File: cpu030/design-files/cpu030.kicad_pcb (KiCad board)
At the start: 4 copper layers, 106 parts, among them J101 Reset, J102 SYSCTL JTAG, J103 NMI, J201 DRAM0SZ, J202 DRAM0 JTAG, J301 UART0 FTDI, J302 UART1 FTDI, J303 UART1, J304 UART0, SW101 Reset, SW102 NMI, U101 MC68030RC, U102 ATF1508AS, U103 MC74ACT05DG, U104 DS1813, U105 SST39SF040 (E), U106 SST39SF040 (O), U107 MC68882, U108 GAL22V10, U109 MC74ACT05DG, U110 DS1813, U201 ATF1508AS, U202 CY7C1061GE (U16), U203 CY7C1061GE (L16), U204 SIMM72-0A, U205 SIMM72-0B, U206 MC74ACT05DG, U301 TL16C2552, Y101 50MHz, Y301 1.8432MHz

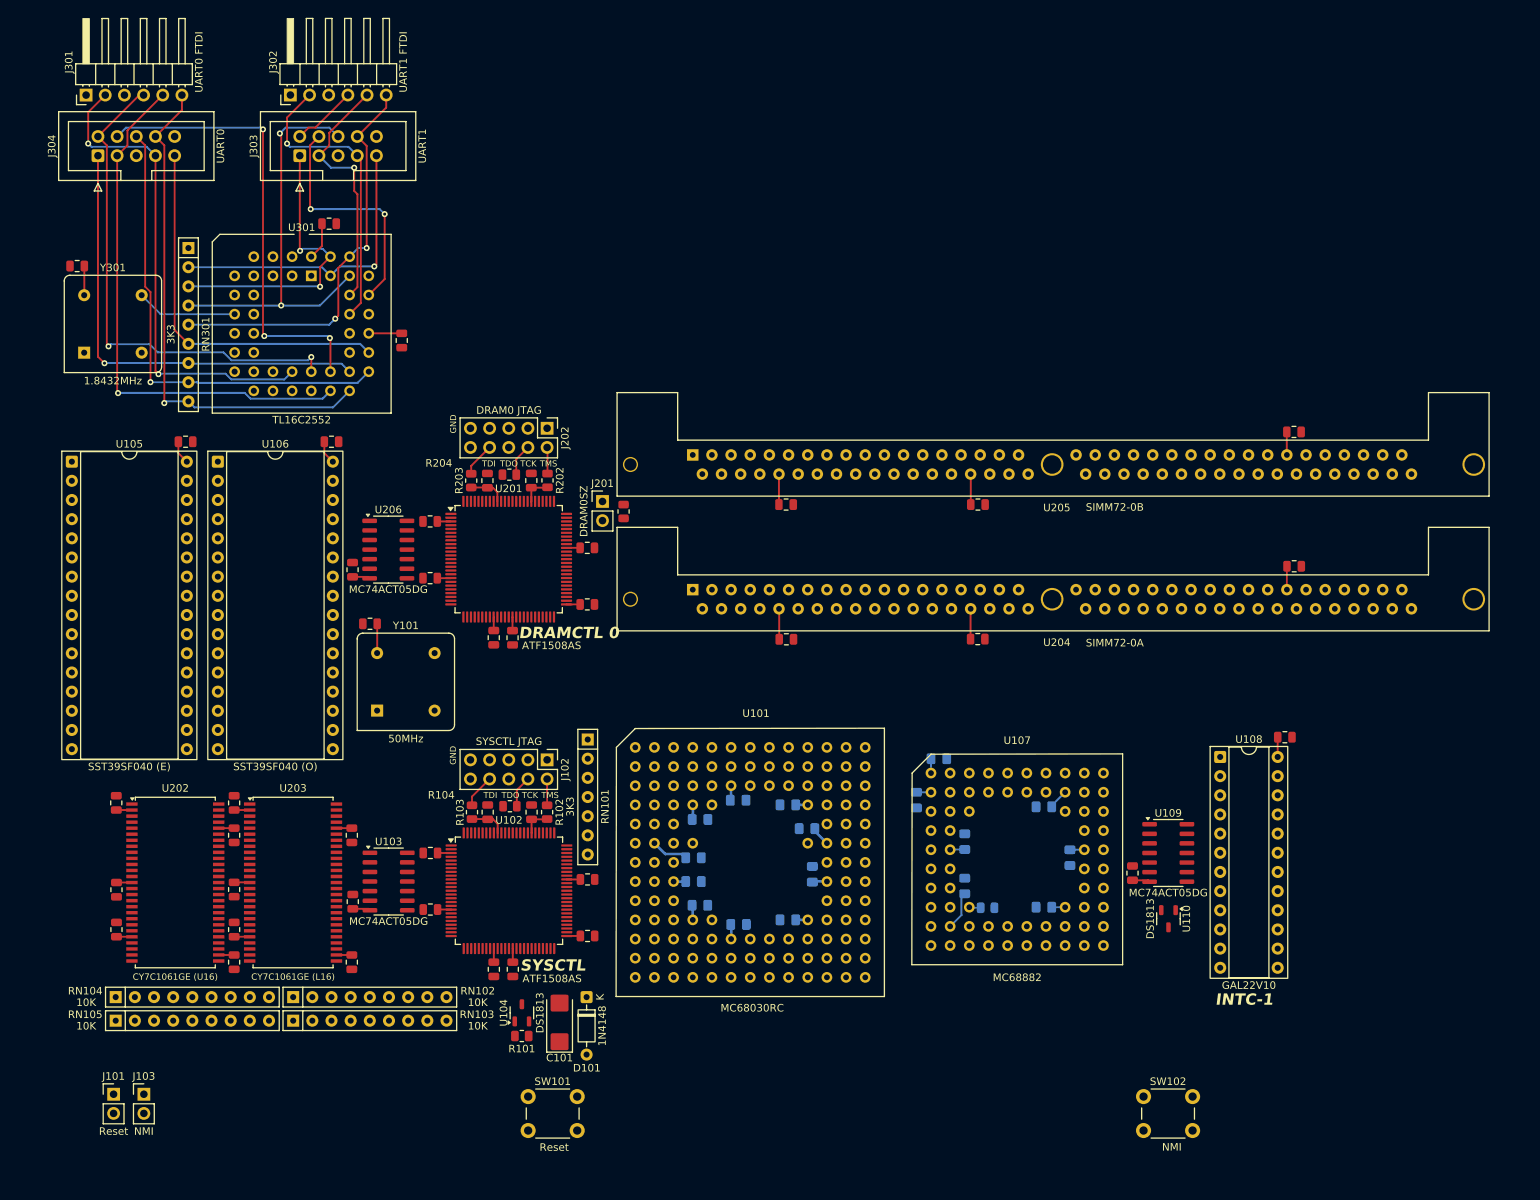
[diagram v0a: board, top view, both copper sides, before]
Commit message: System timer.
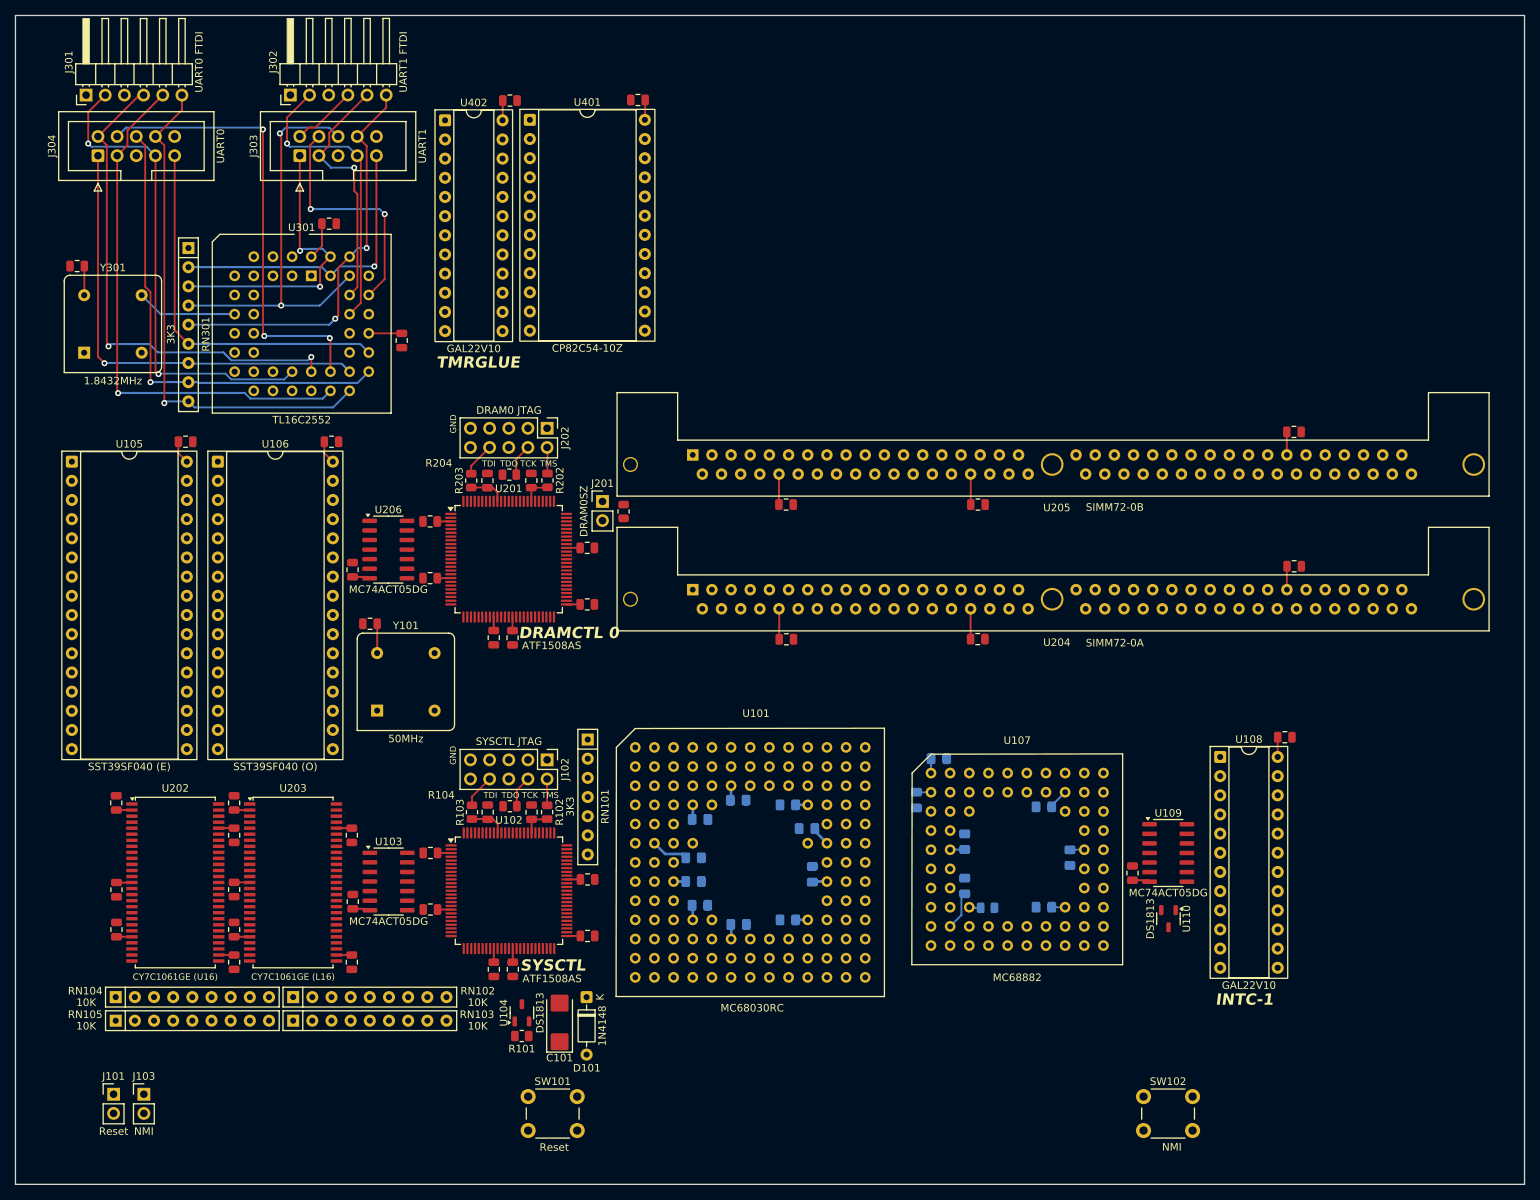
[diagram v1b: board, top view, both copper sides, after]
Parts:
- added C401: 100nF, Capacitor_SMD:C_0805_2012Metric, F.Cu at (228.7, 95.6)
- added C402: 100nF, Capacitor_SMD:C_0805_2012Metric, F.Cu at (211.8, 95.7)
- added U401: CP82C54-10Z, Package_DIP:DIP-24_W15.24mm_Socket, F.Cu at (214.4, 98.2)
- added U402: GAL22V10, Package_DIP:DIP-24_W7.62mm_Socket, F.Cu at (203.2, 98.3)
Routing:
- net +5V: track 154.8 -> 160.1 mm
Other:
- board outline added: 200 x 154.9 mm
- board text added: "TMRGLUE"

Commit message: Eliminate the external D-FF clocking on INTC-1; use the same trick with /DS as we do on TMRGLUE.
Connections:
- U108 pad 1: Net-(U108-I1/CLK) -> ~{DS}
- U108 pad 13: ~{DS} -> RnW
- U108 pad 14: RnW -> unconnected-(U108-IO1-Pad14)
- U108 pad 23: Net-(U108-I1/CLK) -> unconnected-(U108-IO10-Pad23)
- U109 pad 5: GND -> TMR_O0
- U109 pad 6: unconnected-(U109-Pad6) -> ~{INT6}
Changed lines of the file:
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@@
 	(net 251 "Net-(U107-A0)")
 	(net 252 "~{INT5}")
-	(net 253 "Net-(U108-I1{slash}CLK)")
-	(net 254 "~{INT1}")
-	(net 255 "~{INT7}")
-	(net 256 "~{INT6}")
-	(net 257 "~{INT2}")
-	(net 258 "~{INT4}")
-	(net 259 "~{INT3}")
-	(net 260 "unconnected-(U108-IO9-Pad22)")
-	(net 261 "unconnected-(U109-Pad10)")
-	(net 262 "unconnected-(U109-Pad8)")
-	(net 263 "unconnected-(U109-Pad6)")
-	(net 264 "unconnected-(U109-Pad12)")
-	(net 265 "Net-(U401-OUT0)")
-	(net 266 "Net-(U401-G2)")
-	(net 267 "Net-(U401-~{CS})")
-	(net 268 "Net-(U401-OUT2)")
-	(net 269 "Net-(U401-G1)")
-	(net 270 "Net-(U401-OUT1)")
-	(net 271 "Net-(U401-G0)")
-	(net 272 "unconnected-(U402-I8-Pad8)")
-	(net 273 "unconnected-(U402-I11-Pad11)")
-	(net 274 "unconnected-(U402-I9-Pad9)")
-	(net 275 "TMR_O2")
-	(net 276 "unconnected-(U402-I10-Pad10)")
-	(net 277 "TMR_O0")
-	(net 278 "TMR_O1")
+	(net 253 "~{INT1}")
+	(net 254 "~{INT7}")
+	(net 255 "~{INT6}")
+	(net 256 "~{INT2}")
+	(net 257 "~{INT4}")
+	(net 258 "~{INT3}")
+	(net 259 "unconnected-(U108-IO9-Pad22)")
+	(net 260 "unconnected-(U109-Pad10)")
+	(net 261 "unconnected-(U109-Pad8)")
+	(net 262 "unconnected-(U109-Pad12)")
+	(net 263 "Net-(U401-OUT0)")
+	(net 264 "Net-(U401-G2)")
+	(net 265 "Net-(U401-~{CS})")
+	(net 266 "Net-(U401-OUT2)")
+	(net 267 "Net-(U401-G1)")
+	(net 268 "Net-(U401-OUT1)")
+	(net 269 "Net-(U401-G0)")
+	(net 270 "unconnected-(U402-I8-Pad8)")
+	(net 271 "unconnected-(U402-I11-Pad11)")
+	(net 272 "unconnected-(U402-I9-Pad9)")
+	(net 273 "TMR_O2")
+	(net 274 "unconnected-(U402-I10-Pad10)")
+	(net 275 "TMR_O0")
+	(net 276 "TMR_O1")
+	(net 277 "unconnected-(U108-IO1-Pad14)")
+	(net 278 "unconnected-(U108-IO10-Pad23)")
 	(footprint "Package_QFP:TQFP-100_14x14mm_P0.5mm"
 		(layer "F.Cu")
@@
 			(layers "*.Cu" "*.Mask")
 			(remove_unused_layers no)
-			(net 265 "Net-(U401-OUT0)")
+			(net 263 "Net-(U401-OUT0)")
 			(pinfunction "I5")
 			(pintype "input")
@@
 			(layers "*.Cu" "*.Mask")
 			(remove_unused_layers no)
-			(net 270 "Net-(U401-OUT1)")
+			(net 268 "Net-(U401-OUT1)")
 			(pinfunction "I6")
 			(pintype "input")
@@
 			(layers "*.Cu" "*.Mask")
 			(remove_unused_layers no)
-			(net 268 "Net-(U401-OUT2)")
+			(net 266 "Net-(U401-OUT2)")
 			(pinfunction "I7")
 			(pintype "input")
@@
 			(layers "*.Cu" "*.Mask")
 			(remove_unused_layers no)
-			(net 272 "unconnected-(U402-I8-Pad8)")
+			(net 270 "unconnected-(U402-I8-Pad8)")
 			(pinfunction "I8")
 			(pintype "input+no_connect")
@@
 			(layers "*.Cu" "*.Mask")
 			(remove_unused_layers no)
-			(net 274 "unconnected-(U402-I9-Pad9)")
+			(net 272 "unconnected-(U402-I9-Pad9)")
 			(pinfunction "I9")
 			(pintype "input+no_connect")
@@
 			(layers "*.Cu" "*.Mask")
 			(remove_unused_layers no)
-			(net 276 "unconnected-(U402-I10-Pad10)")
+			(net 274 "unconnected-(U402-I10-Pad10)")
 			(pinfunction "I10")
 			(pintype "input+no_connect")
@@
 			(layers "*.Cu" "*.Mask")
 			(remove_unused_layers no)
-			(net 273 "unconnected-(U402-I11-Pad11)")
+			(net 271 "unconnected-(U402-I11-Pad11)")
 			(pinfunction "I11")
 			(pintype "input+no_connect")
@@
 			(layers "*.Cu" "*.Mask")
 			(remove_unused_layers no)
-			(net 277 "TMR_O0")
+			(net 275 "TMR_O0")
 			(pinfunction "IO4")
 			(pintype "tri_state")
@@
 			(layers "*.Cu" "*.Mask")
 			(remove_unused_layers no)
-			(net 278 "TMR_O1")
+			(net 276 "TMR_O1")
 			(pinfunction "IO5")
 			(pintype "tri_state")
@@
 			(layers "*.Cu" "*.Mask")
 			(remove_unused_layers no)
-			(net 275 "TMR_O2")
+			(net 273 "TMR_O2")
 			(pinfunction "IO6")
 			(pintype "tri_state")
@@
 			(layers "*.Cu" "*.Mask")
 			(remove_unused_layers no)
-			(net 271 "Net-(U401-G0)")
+			(net 269 "Net-(U401-G0)")
 			(pinfunction "IO7")
 			(pintype "tri_state")
@@
 			(layers "*.Cu" "*.Mask")
 			(remove_unused_layers no)
-			(net 269 "Net-(U401-G1)")
+			(net 267 "Net-(U401-G1)")
 			(pinfunction "IO8")
 			(pintype "tri_state")
@@
 			(layers "*.Cu" "*.Mask")
 			(remove_unused_layers no)
-			(net 266 "Net-(U401-G2)")
+			(net 264 "Net-(U401-G2)")
 			(pinfunction "IO9")
 			(pintype "tri_state")
@@
 			(layers "*.Cu" "*.Mask")
 			(remove_unused_layers no)
-			(net 267 "Net-(U401-~{CS})")
+			(net 265 "Net-(U401-~{CS})")
 			(pinfunction "IO10")
 			(pintype "tri_state")
@@
 			(layers "*.Cu" "*.Mask")
 			(remove_unused_layers no)
-			(net 265 "Net-(U401-OUT0)")
+			(net 263 "Net-(U401-OUT0)")
 			(pinfunction "OUT0")
 			(pintype "output")
@@
 			(layers "*.Cu" "*.Mask")
 			(remove_unused_layers no)
-			(net 271 "Net-(U401-G0)")
+			(net 269 "Net-(U401-G0)")
 			(pinfunction "G0")
 			(pintype "input")
@@
 			(layers "*.Cu" "*.Mask")
 			(remove_unused_layers no)
-			(net 270 "Net-(U401-OUT1)")
+			(net 268 "Net-(U401-OUT1)")
 			(pinfunction "OUT1")
 			(pintype "output")
@@
 			(layers "*.Cu" "*.Mask")
 			(remove_unused_layers no)
-			(net 269 "Net-(U401-G1)")
+			(net 267 "Net-(U401-G1)")
 			(pinfunction "G1")
 			(pintype "input")
@@
 			(layers "*.Cu" "*.Mask")
 			(remove_unused_layers no)
-			(net 266 "Net-(U401-G2)")
+			(net 264 "Net-(U401-G2)")
 			(pinfunction "G2")
 			(pintype "input")
@@
 			(layers "*.Cu" "*.Mask")
 			(remove_unused_layers no)
-			(net 268 "Net-(U401-OUT2)")
+			(net 266 "Net-(U401-OUT2)")
 			(pinfunction "OUT2")
 			(pintype "output")
@@
 			(layers "*.Cu" "*.Mask")
 			(remove_unused_layers no)
-			(net 267 "Net-(U401-~{CS})")
+			(net 265 "Net-(U401-~{CS})")
 			(pinfunction "~{CS}")
 			(pintype "input")
@@
 			(layers "F.Cu" "F.Mask" "F.Paste")
 			(roundrect_rratio 0.25)
-			(net 11 "GND")
+			(net 275 "TMR_O0")
 			(pintype "input")
 		)
@@
 			(layers "F.Cu" "F.Mask" "F.Paste")
 			(roundrect_rratio 0.25)
-			(net 263 "unconnected-(U109-Pad6)")
-			(pintype "open_collector+no_connect")
+			(net 255 "~{INT6}")
+			(pintype "open_collector")
 		)
 		(pad "7" smd roundrect
@@
 			(layers "F.Cu" "F.Mask" "F.Paste")
 			(roundrect_rratio 0.25)
-			(net 262 "unconnected-(U109-Pad8)")
+			(net 261 "unconnected-(U109-Pad8)")
 			(pintype "open_collector+no_connect")
 		)
@@
 			(layers "F.Cu" "F.Mask" "F.Paste")
 			(roundrect_rratio 0.25)
-			(net 261 "unconnected-(U109-Pad10)")
+			(net 260 "unconnected-(U109-Pad10)")
 			(pintype "open_collector+no_connect")
 		)
@@
 			(layers "F.Cu" "F.Mask" "F.Paste")
 			(roundrect_rratio 0.25)
-			(net 264 "unconnected-(U109-Pad12)")
+			(net 262 "unconnected-(U109-Pad12)")
 			(pintype "open_collector+no_connect")
 		)
@@
 			(layers "*.Cu" "*.Mask")
 			(remove_unused_layers no)
-			(net 255 "~{INT7}")
+			(net 254 "~{INT7}")
 			(pinfunction "1")
 			(pintype "passive")
@@
 			(layers "*.Cu" "*.Mask")
 			(remove_unused_layers no)
-			(net 255 "~{INT7}")
+			(net 254 "~{INT7}")
 			(pinfunction "1")
 			(pintype "passive")
@@
 			(remove_unused_layers no)
 			(roundrect_rratio 0.15625)
-			(net 253 "Net-(U108-I1{slash}CLK)")
+			(net 86 "~{DS}")
 			(pinfunction "I1/CLK")
 			(pintype "input")
@@
 			(layers "*.Cu" "*.Mask")
 			(remove_unused_layers no)
-			(net 254 "~{INT1}")
+			(net 253 "~{INT1}")
 			(pinfunction "I2")
 			(pintype "input")
@@
 			(layers "*.Cu" "*.Mask")
 			(remove_unused_layers no)
-			(net 257 "~{INT2}")
+			(net 256 "~{INT2}")
 			(pinfunction "I3")
 			(pintype "input")
@@
 			(layers "*.Cu" "*.Mask")
 			(remove_unused_layers no)
-			(net 259 "~{INT3}")
+			(net 258 "~{INT3}")
 			(pinfunction "I4")
 			(pintype "input")
@@
 			(layers "*.Cu" "*.Mask")
 			(remove_unused_layers no)
-			(net 258 "~{INT4}")
+			(net 257 "~{INT4}")
 			(pinfunction "I5")
 			(pintype "input")
@@
 			(layers "*.Cu" "*.Mask")
 			(remove_unused_layers no)
-			(net 256 "~{INT6}")
+			(net 255 "~{INT6}")
 			(pinfunction "I7")
 			(pintype "input")
@@
 			(layers "*.Cu" "*.Mask")
 			(remove_unused_layers no)
-			(net 255 "~{INT7}")
+			(net 254 "~{INT7}")
 			(pinfunction "I8")
 			(pintype "input")
@@
 			(layers "*.Cu" "*.Mask")
 			(remove_unused_layers no)
-			(net 86 "~{DS}")
+			(net 28 "RnW")
 			(pinfunction "I12")
 			(pintype "input")
@@
 			(layers "*.Cu" "*.Mask")
 			(remove_unused_layers no)
-			(net 28 "RnW")
+			(net 277 "unconnected-(U108-IO1-Pad14)")
 			(pinfunction "IO1")
-			(pintype "tri_state")
+			(pintype "tri_state+no_connect")
 		)
 		(pad "15" thru_hole circle
@@
 			(layers "*.Cu" "*.Mask")
 			(remove_unused_layers no)
-			(net 260 "unconnected-(U108-IO9-Pad22)")
+			(net 259 "unconnected-(U108-IO9-Pad22)")
 			(pinfunction "IO9")
 			(pintype "tri_state+no_connect")
@@
 			(layers "*.Cu" "*.Mask")
 			(remove_unused_layers no)
-			(net 253 "Net-(U108-I1{slash}CLK)")
+			(net 278 "unconnected-(U108-IO10-Pad23)")
 			(pinfunction "IO10")
-			(pintype "tri_state")
+			(pintype "tri_state+no_connect")
 		)
 		(pad "24" thru_hole circle
@@
 			(layers "*.Cu" "*.Mask")
 			(remove_unused_layers no)
-			(net 255 "~{INT7}")
+			(net 254 "~{INT7}")
 			(pinfunction "Pin_1")
 			(pintype "passive")
@@
 			(layers "F.Cu" "F.Mask" "F.Paste")
 			(roundrect_rratio 0.25)
-			(net 255 "~{INT7}")
+			(net 254 "~{INT7}")
 			(pinfunction "~{RST}")
 			(pintype "open_collector")
